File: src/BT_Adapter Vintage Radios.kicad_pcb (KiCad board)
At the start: 2 copper layers, 60 x 23.8 mm, 18 parts, among them Q1 IRF620N, U1 PS2561, U2 LM7805

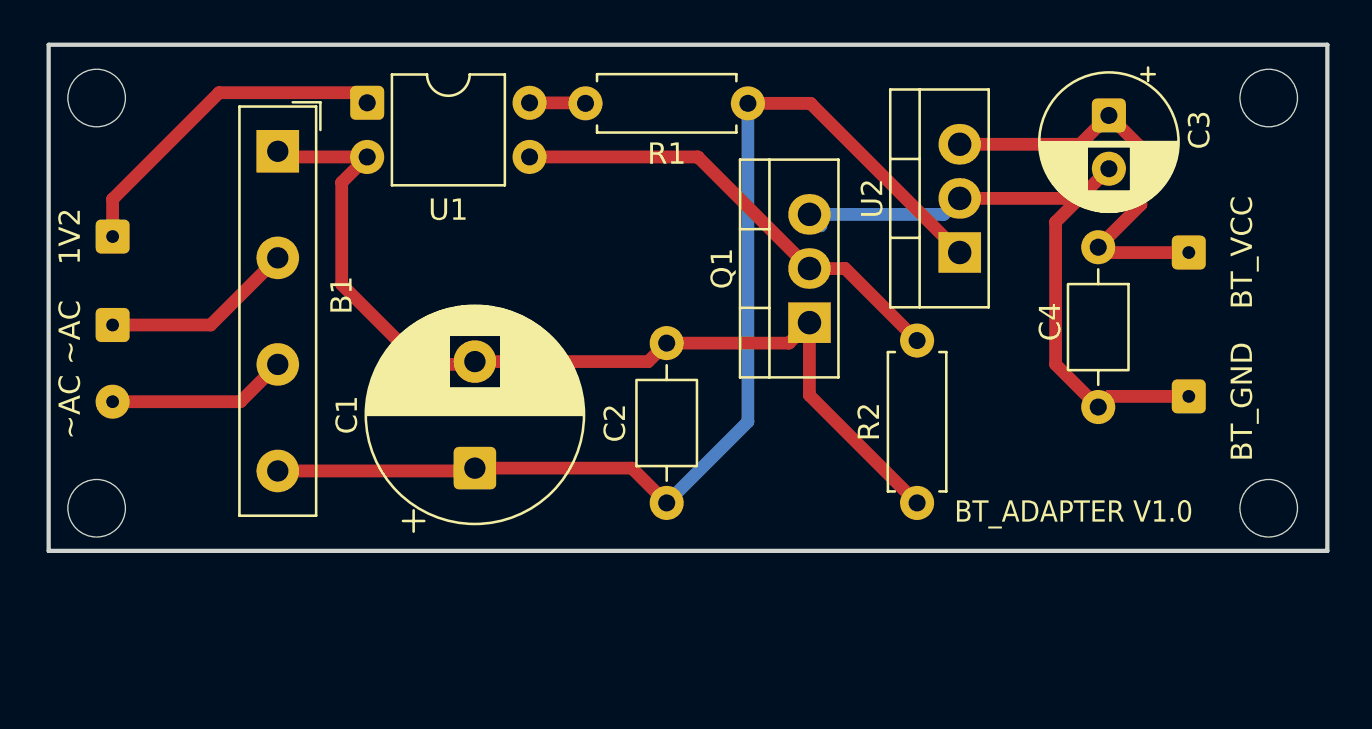
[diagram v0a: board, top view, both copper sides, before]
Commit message: Minor improvements
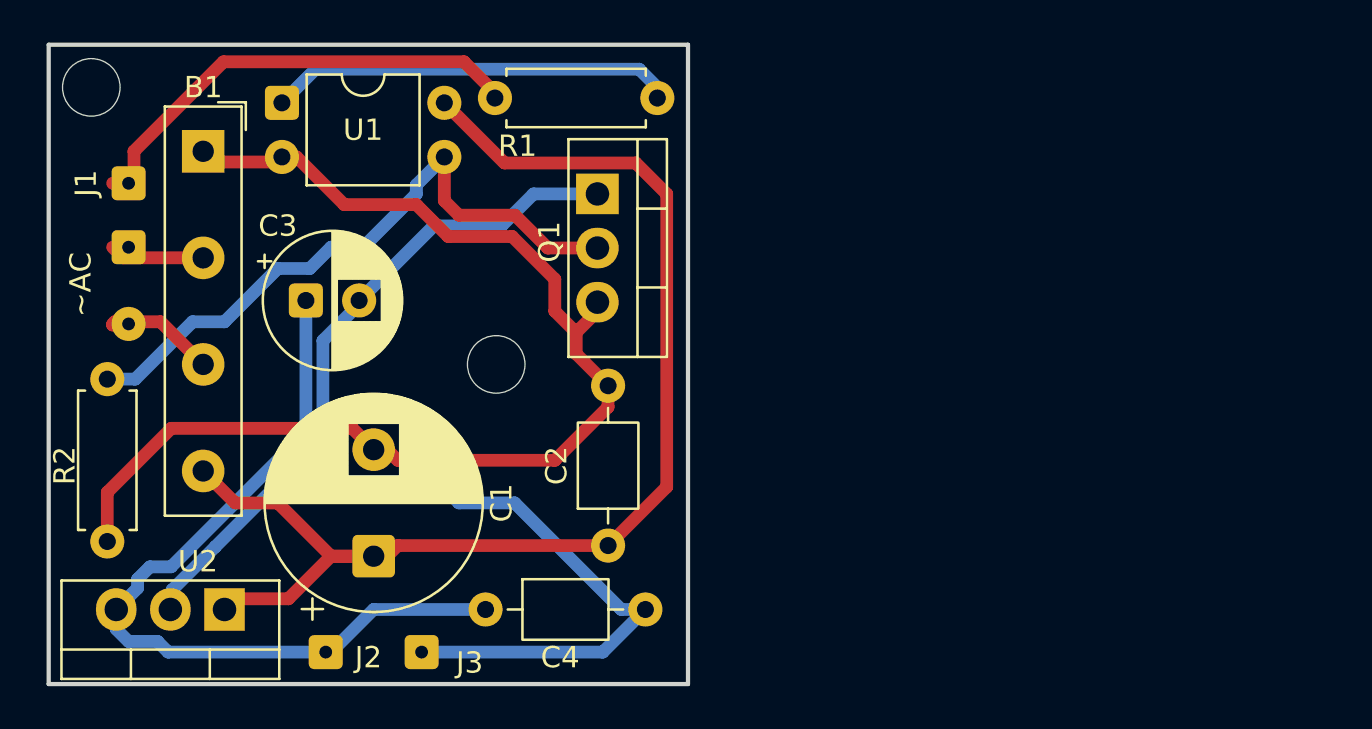
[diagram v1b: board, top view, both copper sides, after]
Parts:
- removed the REF** at (172.5, 73.5)
- removed the REF** at (117.5, 73.5)
- removed the REF** at (172.5, 92.8)
- removed the REF** at (117.5, 92.8)
- added REF**: MountingHole_2.7mm_M2.5, MountingHole:MountingHole_2.7mm_M2.5, F.Cu at (136.2, 86.0)
- added REF**: MountingHole_2.7mm_M2.5, MountingHole:MountingHole_2.7mm_M2.5, F.Cu at (117.2, 73.0)
- J1: renamed from 1V2; value 1V2_SEP -> 1V2_SEPARATED
- R1: value 1k -> 220
- moved J2 44.6 mm to (128.2, 99.5)
- moved C3 38.7 mm to (127.3, 83.0), turned to 0 degrees
- moved U2 38.4 mm to (123.5, 97.5), turned to 180 degrees
- moved R2 38.0 mm to (118.0, 86.7)
- moved J3 37.9 mm to (132.8, 99.5)
- moved C4 33.4 mm to (135.8, 97.5), turned to 0 degrees
- moved R1 11.9 mm to (136.2, 73.5), turned to 0 degrees
- moved Q1 11.6 mm to (141.0, 78.0), turned to -90 degrees
- moved C1 6.30 mm to (130.5, 95.0)
- moved U1 4.00 mm to (126.2, 73.7)
- moved I1 3.73 mm to (119.0, 80.5)
- moved B1 3.50 mm to (122.5, 76.0)
- moved C2 3.40 mm to (141.5, 94.5)
- moved J1 2.61 mm to (119.0, 77.5)
- renumbered ~AC to I1, BT_VCC to J2, BT_GND to J3
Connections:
- Q1 pad 1: GND -> Net-(J3-Pin_1)
- Q1 pad 3: Net-(J3-Pin_1) -> GND
- R1 pad 1: VCC -> Net-(J1-Pin_1)
- U1 pad 1: Net-(J1-Pin_1) -> Net-(R1-Pad2)
- U1 pad 4: Net-(R1-Pad2) -> VCC
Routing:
- net Net-(J3-Pin_1): track 31.2 -> 61.8 mm
- net Net-(J2-Pin_1): track 20.4 -> 38.3 mm
- net Net-(R1-Pad2): track 2.64 -> 19.0 mm
- net GND: track 46.4 -> 56.8 mm
- net Net-(Q1-G): track 21.8 -> 30.5 mm
- net VCC: track 52.1 -> 58.8 mm
- net Net-(B1-Pad2): track 10.5 -> 4.46 mm
- net Net-(J1-Pin_1): track 16.6 -> 21.6 mm
- net Net-(B1-Pad3): track 8.47 -> 5.90 mm
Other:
- board size 60 x 23.8 mm -> 30 x 30 mm
- board text removed: "BT_ADAPTER V1.0"
